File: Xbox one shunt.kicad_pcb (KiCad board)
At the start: 2 copper layers, 13 x 13.2 mm, 13 parts, among them U1 INA181A1-Q1, U2 TLV3201AIDCKR

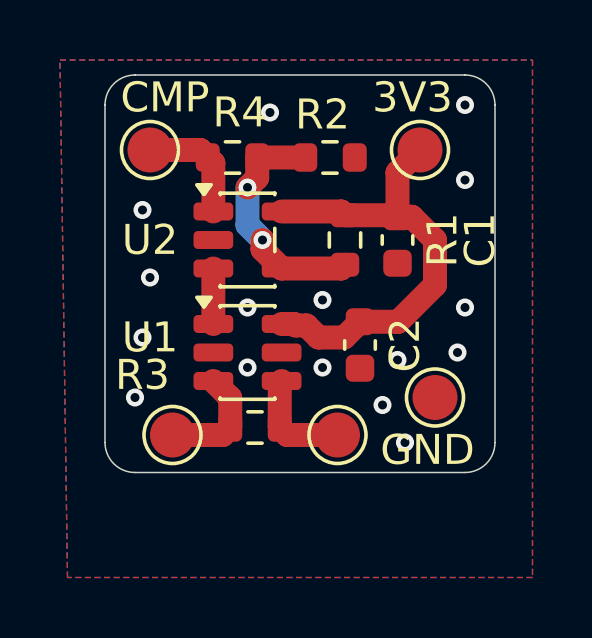
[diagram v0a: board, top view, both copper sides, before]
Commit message: quick fixes
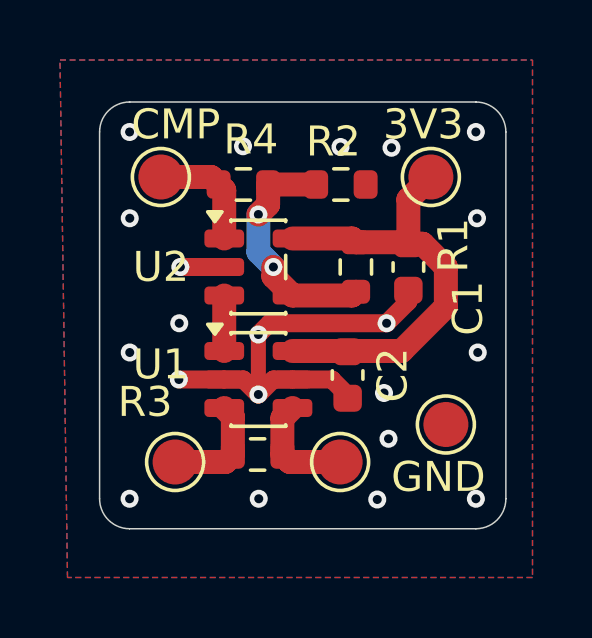
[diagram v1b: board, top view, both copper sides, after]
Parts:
- moved C2 1.08 mm to (96.6, 103.8)
- moved 3V3 0.97 mm to (99.4, 97.2)
- moved C1 0.97 mm to (98.6, 100.2)
- moved CMP 0.97 mm to (90.4, 97.2)
- moved GND 0.97 mm to (99.9, 105.4)
- moved R1 0.97 mm to (96.9, 100.2)
- moved R2 0.97 mm to (96.4, 97.4)
- moved R4 0.97 mm to (93.1, 97.4)
- moved U1 0.97 mm to (93.6, 103.9)
- moved U2 0.97 mm to (93.6, 100.2)
- moved R3 0.90 mm to (93.6, 106.4)
- moved TP2 0.90 mm to (90.8, 106.7)
- moved TP3 0.90 mm to (96.3, 106.7)
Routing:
- net GND: track 0.00 -> 15.5 mm, vias 16 -> 21
- net +3.3V: track 15.6 -> 15.0 mm
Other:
- board size 13 x 13.2 mm -> 13.5 x 14.2 mm
